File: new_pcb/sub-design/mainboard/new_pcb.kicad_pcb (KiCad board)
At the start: 2 copper layers, 73 parts, among them P1 USB_OTG, P2 USB_OTG, U1 STM32F407VGTx, U2 H28, U3 FT232RL, U4 LM317_SOT223, Y1 24MHz, Y2 32kHz

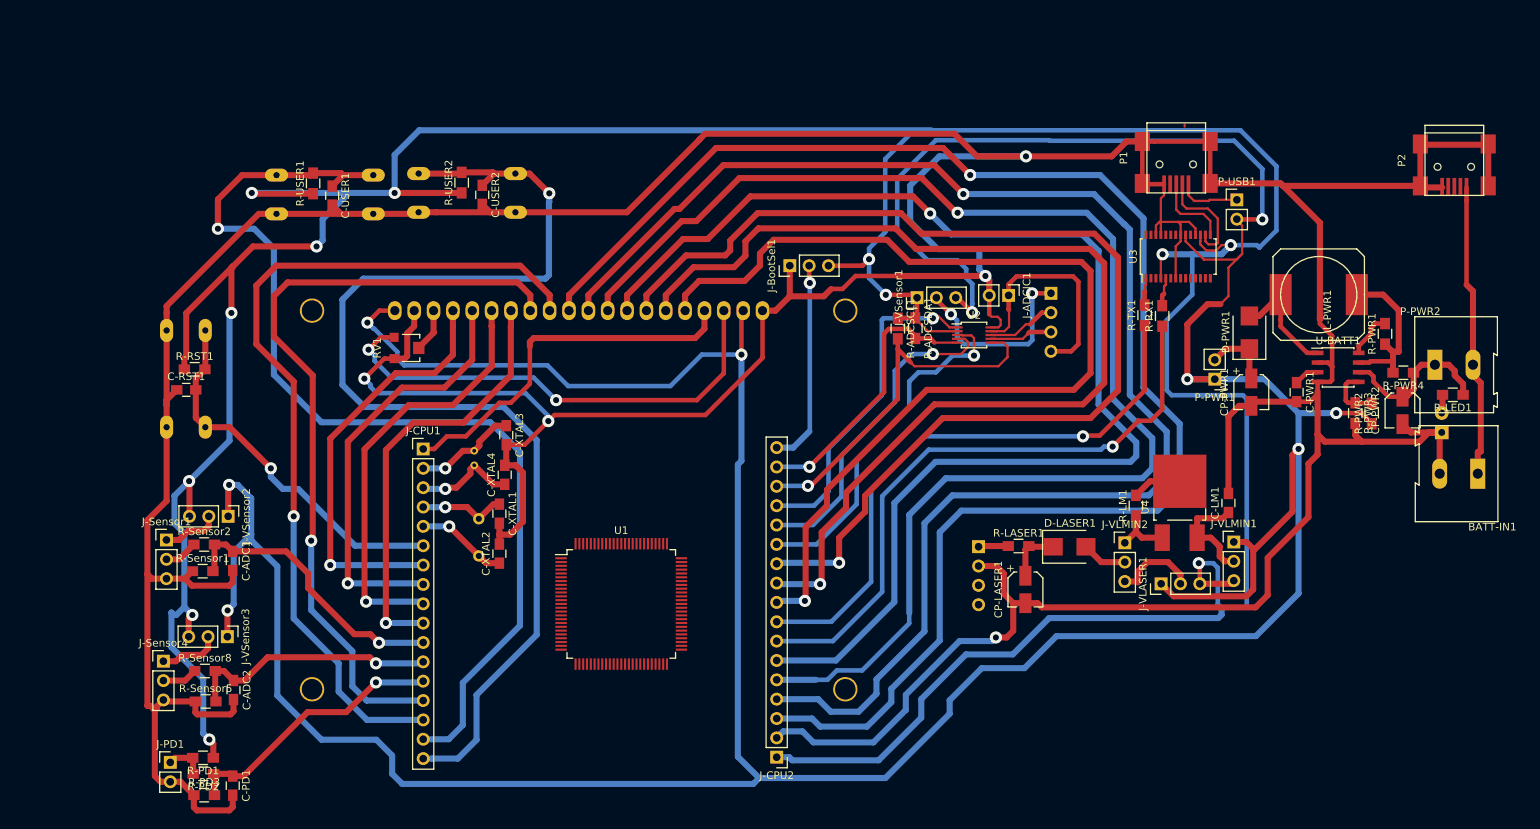
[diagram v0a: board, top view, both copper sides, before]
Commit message: new design
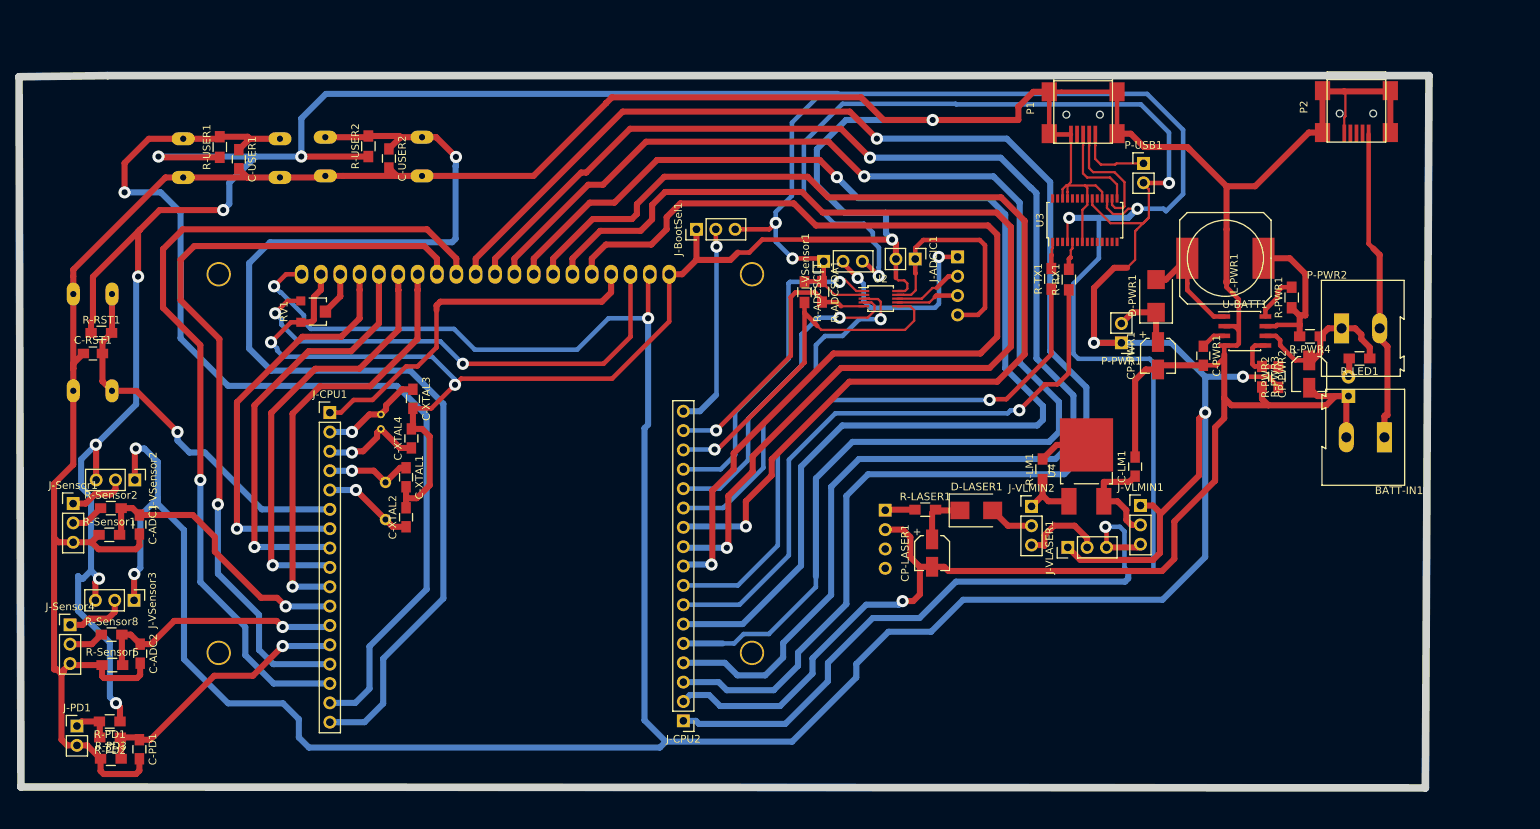
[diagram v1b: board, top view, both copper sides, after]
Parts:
- removed U1: STM32F407VGTx, Housings_QFP:LQFP-100_14x14mm_Pitch0.5mm
- moved P2 14.6 mm to (231.8, 54.6)
- moved P1 13.9 mm to (195.9, 54.7)
- moved C-ADC1 13.1 mm to (72.1, 108.7)
- moved C-LM1 13.1 mm to (202.8, 101.1)
- moved C-PD1 13.1 mm to (72.1, 138.2)
- moved C-USER2 13.1 mm to (104.8, 60.7)
- moved C-XTAL3 13.1 mm to (108.0, 92.2)
- moved C-XTAL4 13.1 mm to (107.8, 97.4)
- moved CP-LASER1 13.1 mm to (176.1, 112.5)
- moved CP-PWR2 13.1 mm to (225.6, 89.0)
- moved D-LASER1 13.1 mm to (181.9, 106.9)
- moved D-PWR1 13.1 mm to (205.5, 78.7)
- moved DS1 13.1 mm to (93.4, 75.9)
- moved J-ADCIC1 13.1 mm to (173.9, 73.9)
- moved J-BootSel1 13.1 mm to (145.2, 70.0)
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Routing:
- net GND: track 736.0 -> 740.6 mm
- net Net-(BATT-IN1-Pad1): track 38.7 -> 41.2 mm
- net Net-(P1-Pad2): track 14.0 -> 15.8 mm
- net Net-(P-USB1-Pad1): track 8.17 -> 9.93 mm
- net Net-(P1-Pad3): track 10.3 -> 12.0 mm
- added copper zone on B.Cu, net (none)
- added copper zone on F.Cu, net (none)
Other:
- board outline added: 185.1 x 93.5 mm

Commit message: progress
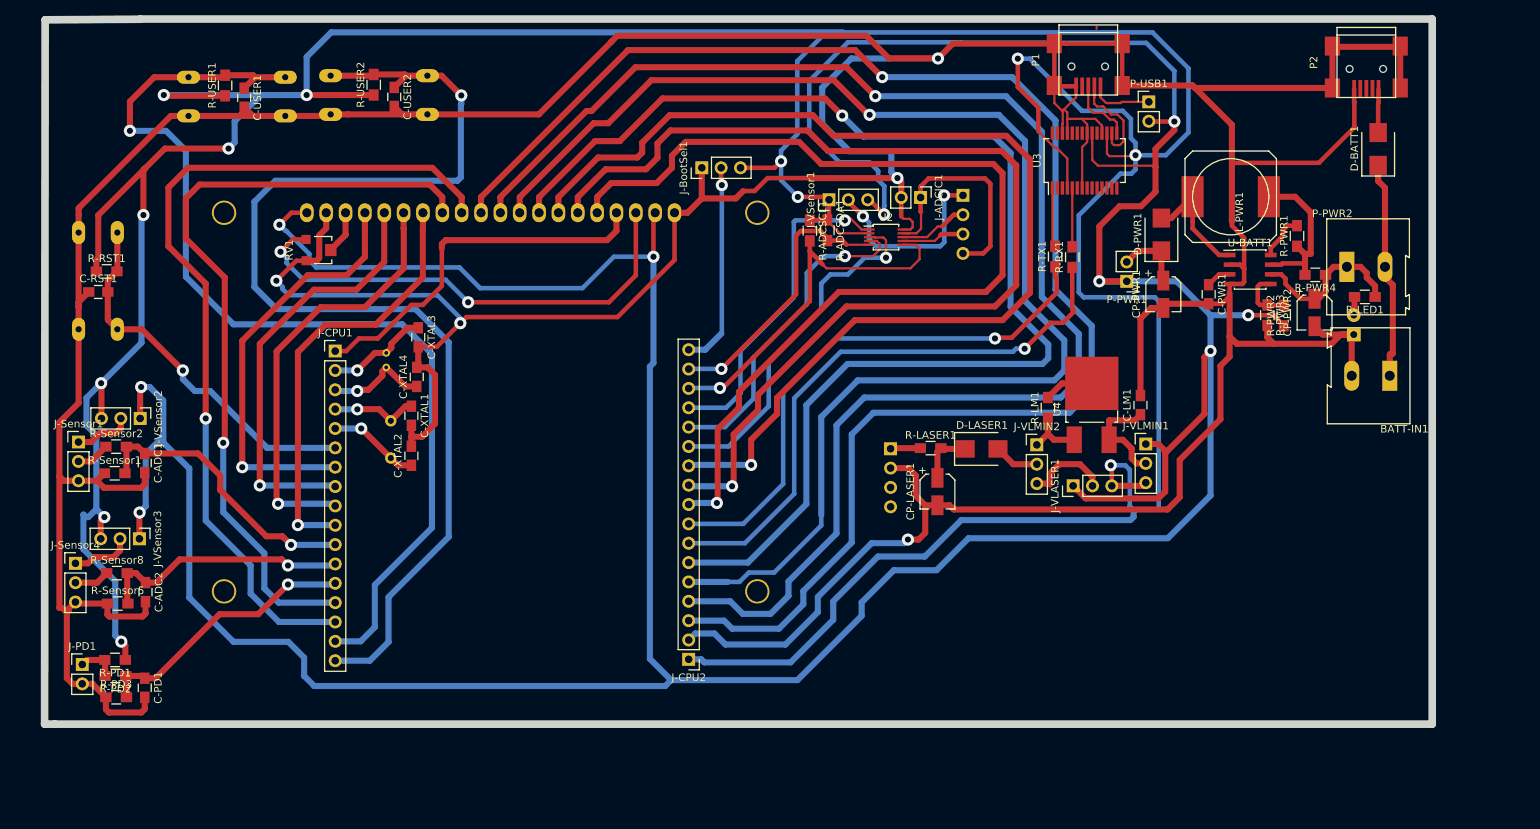
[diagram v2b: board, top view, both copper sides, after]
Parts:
- added D-BATT1: D, Diodes_SMD:D_SMB_Standard, F.Cu at (234.7, 59.4)
- U3: footprint Housings_SSOP:TSSOP-28_4.4x9.7mm_Pitch0.65mm -> Housings_SSOP:SSOP-28_5.3x10.2mm_Pitch0.65mm
- moved J-PD1 8.11 mm to (64.6, 127.1)
- moved R-PD2 8.11 mm to (68.9, 128.6)
- moved C-PWR1 8.11 mm to (212.4, 78.5)
- moved J-ADCIC1 8.11 mm to (174.6, 65.8)
- moved J-CPU2 8.11 mm to (144.2, 126.4)
- moved J-LDMOUNT1 8.11 mm to (170.7, 98.8)
- moved J-SENMOUNT1 8.11 mm to (180.2, 65.5)
- moved J-VLMIN1 8.11 mm to (204.2, 98.2)
- moved P-PWR1 8.11 mm to (201.7, 76.8)
- moved R-LASER1 8.11 mm to (175.9, 98.7)
- moved R-LED1 8.11 mm to (232.9, 78.8)
- moved R-PWR1 8.11 mm to (224.0, 70.8)
- moved R-PWR2 8.11 mm to (222.3, 81.3)
- moved R-PWR4 8.11 mm to (226.4, 76.0)
- moved BATT-IN1 8.11 mm to (236.2, 89.2)
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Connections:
- P2 pad 1: Net-(BATT-IN1-Pad1) -> Net-(D-BATT1-Pad2)
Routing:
- net VDD: track 506.0 -> 540.9 mm
- net GND: track 740.6 -> 763.5 mm
- net Net-(BATT-IN1-Pad1): track 41.2 -> 28.8 mm
- net Net-(D-BATT1-Pad2): track 0.00 -> 5.67 mm
- net /TX: track 76.5 -> 71.4 mm
- net /RX: track 81.5 -> 76.5 mm
- net VCC: track 537.8 -> 542.1 mm
- net Net-(R-TX1-Pad2): track 3.57 -> 7.79 mm
- net Net-(R-RX1-Pad2): track 3.83 -> 7.73 mm
- net Net-(P1-Pad3): track 12.0 -> 8.76 mm
- net Net-(P1-Pad2): track 15.8 -> 12.9 mm
- net Net-(P-USB1-Pad1): track 9.93 -> 8.17 mm
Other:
- board size 185.1 x 93.5 mm -> 182.2 x 92.6 mm
